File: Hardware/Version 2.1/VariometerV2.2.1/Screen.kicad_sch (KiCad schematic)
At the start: 20 parts, among them J4 FFC24/0.5MM, Q3 AO3400A

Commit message: Finish PCB
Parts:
- J4: LCSC Part C202112 -> C519265
- L3, R34: LCSC Part (none) -> 0
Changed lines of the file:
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@@
       (effects (font (size 1.27 1.27)) (justify left top) hide)
     )
-    (property "LCSC Part" "" (at 81.28 95.25 0)
+    (property "LCSC Part" "0" (at 81.28 95.25 0)
       (effects (font (size 1.27 1.27)) hide)
     )
@@
       (effects (font (size 1.27 1.27)) hide)
     )
-    (property "LCSC Part" "" (at 104.14 72.39 0)
+    (property "LCSC Part" "0" (at 104.14 72.39 0)
       (effects (font (size 1.27 1.27)) hide)
     )
@@
       (effects (font (size 1.27 1.27)) hide)
     )
-    (property "LCSC Part" "C202112" (at 215.9 71.12 0)
+    (property "LCSC Part" "C519265" (at 215.9 71.12 0)
       (effects (font (size 1.27 1.27)) hide)
     )

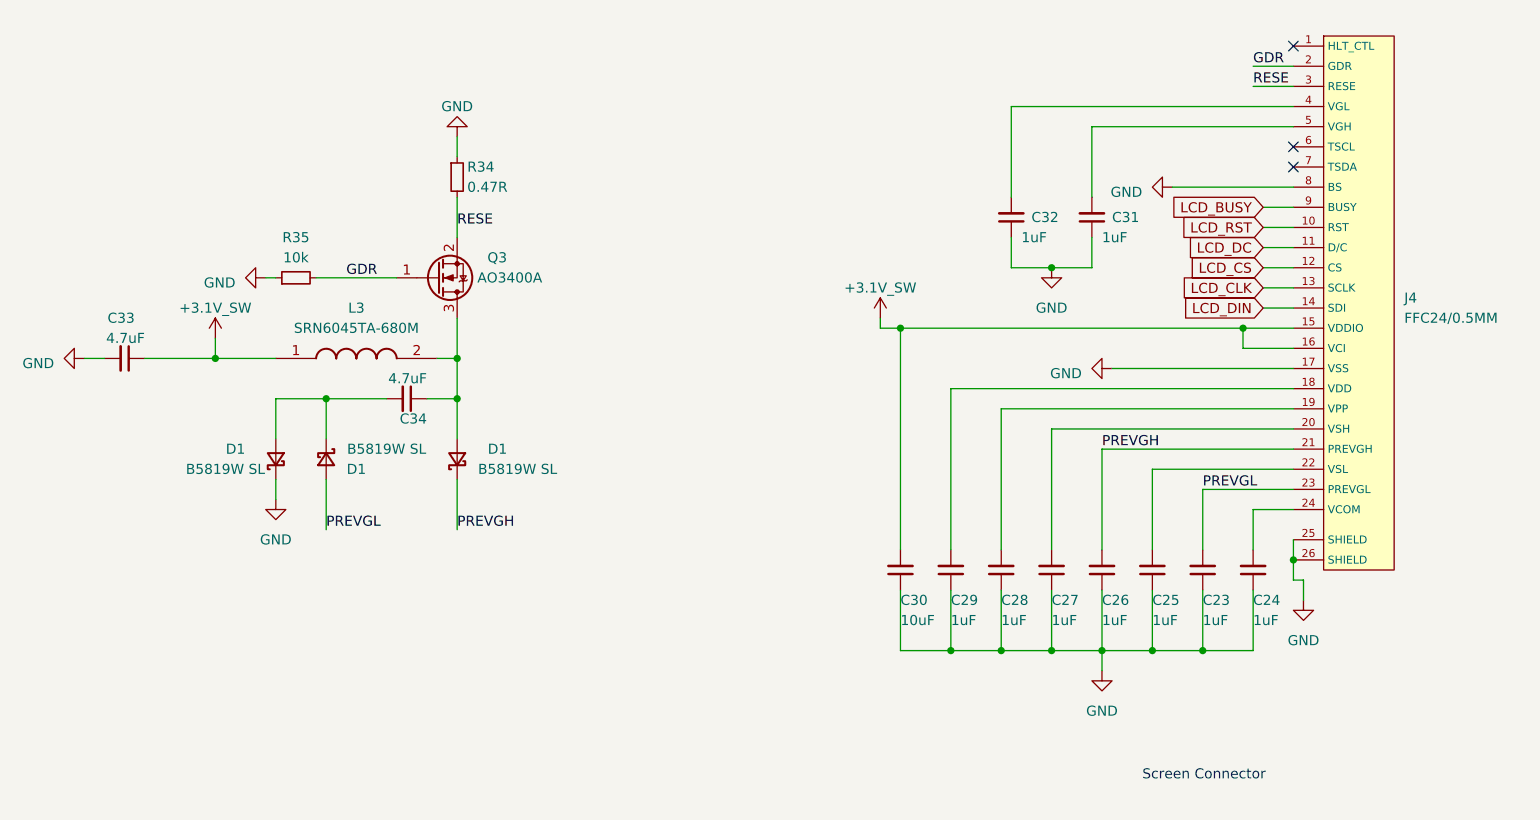
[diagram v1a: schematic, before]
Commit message: Fix Screen Connector PCB
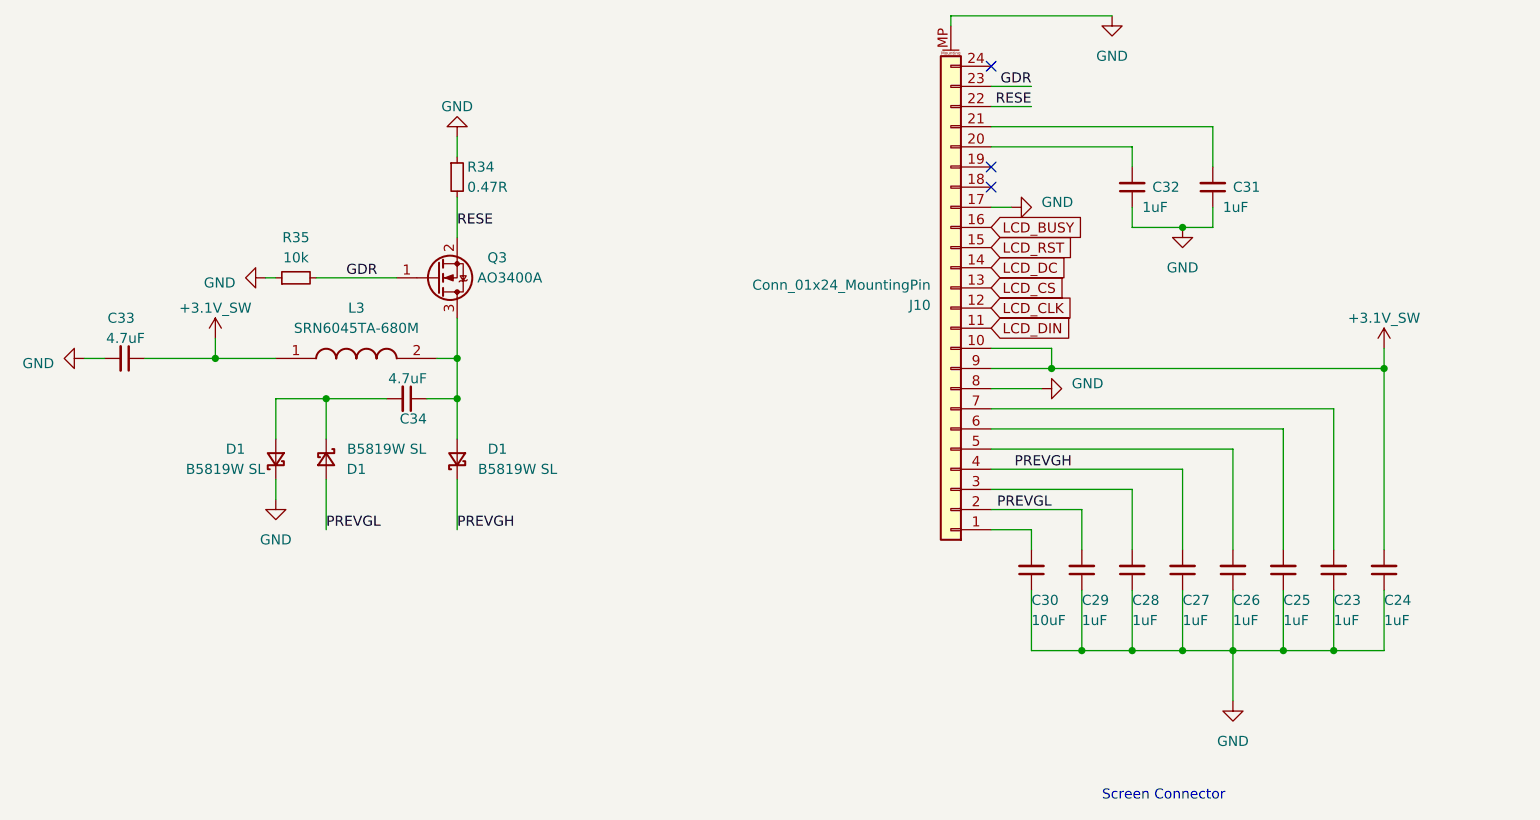
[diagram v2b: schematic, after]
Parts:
- removed J4: FFC24/0.5MM, MainLibrary:FH12-24S-0.5SH_55_, symbol Main_LibraryVario:FFC24/0.5MM
- added J10: Conn_01x24_MountingPin, Connector_FFC-FPC:Hirose_FH12-24S-0.5SH_1x24-1MP_P0.50mm_Horizontal, symbol Connector_Generic_MountingPin:Conn_01x24_MountingPin
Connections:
- net +3.1V_SW: now also C24.2, J10.10 (Pin_10), J10.9 (Pin_9); no longer C30.2
- net GDR: now also J10.23 (Pin_23)
- net GND: now also J10.17 (Pin_17), J10.8 (Pin_8), J10.MP (MountPin)
- net LCD_BUSY: now also J10.16 (Pin_16)
- net LCD_CLK: now also J10.12 (Pin_12)
- net LCD_CS: now also J10.13 (Pin_13)
- net LCD_DC: now also J10.14 (Pin_14)
- net LCD_DIN: now also J10.11 (Pin_11)
- net LCD_RST: now also J10.15 (Pin_15)
- net PREVGH: now also C27.2, J10.4 (Pin_4); no longer C26.2
- net PREVGL: now also C29.2, J10.2 (Pin_2); no longer C23.2
- net RESE: now also J10.22 (Pin_22)
- net at C31.2: now also J10.21 (Pin_21)
- net at C28.2: now also J10.3 (Pin_3)
- net at C25.2: now also J10.6 (Pin_6)
- net at C32.2: now also J10.20 (Pin_20)
- new net: C30.2, J10.1 (Pin_1)
- new net: C26.2, J10.5 (Pin_5)
- new net: C23.2, J10.7 (Pin_7)
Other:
- moved on the sheet: C23, C24, C25, C26, C27, C28, C29, C30, C31, C32
